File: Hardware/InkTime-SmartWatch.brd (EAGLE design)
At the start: 46 x 35 mm, 105 parts, among them IC1 BQ25180YBGR, IC2 DRV2605YZFR, IC3 BMA421, IC9 RT6160AWSC, J1 503480-2400, J2 TC2030-IDC, J4 KH-TYPE-C-16P, Q1 20V/4.2A/52mΩ/1.4W, Q3 SI1308EDL-T1-GE3, U1 NRF52840_QF, U3 MAX17048G+T10, X1 32MHz, X2 32.768kHz

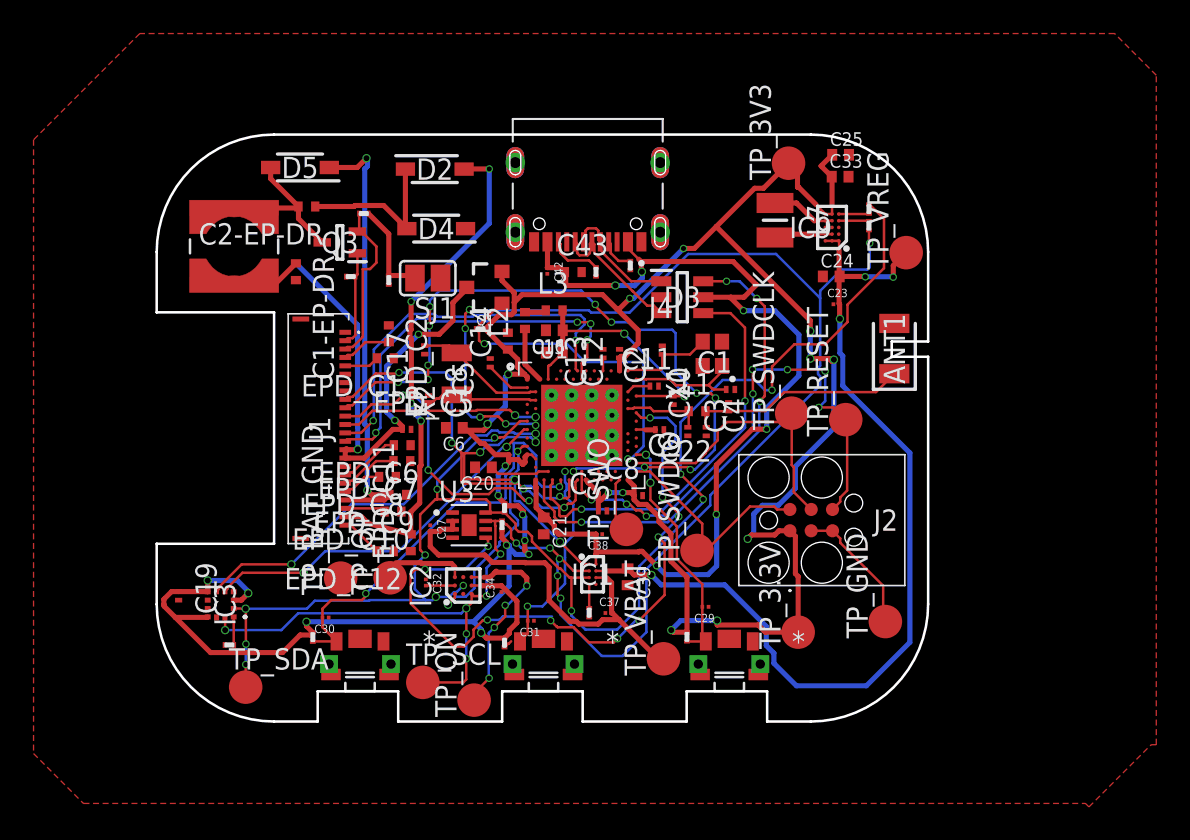
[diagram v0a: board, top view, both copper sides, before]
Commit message: Varianta finala de PCB 2D
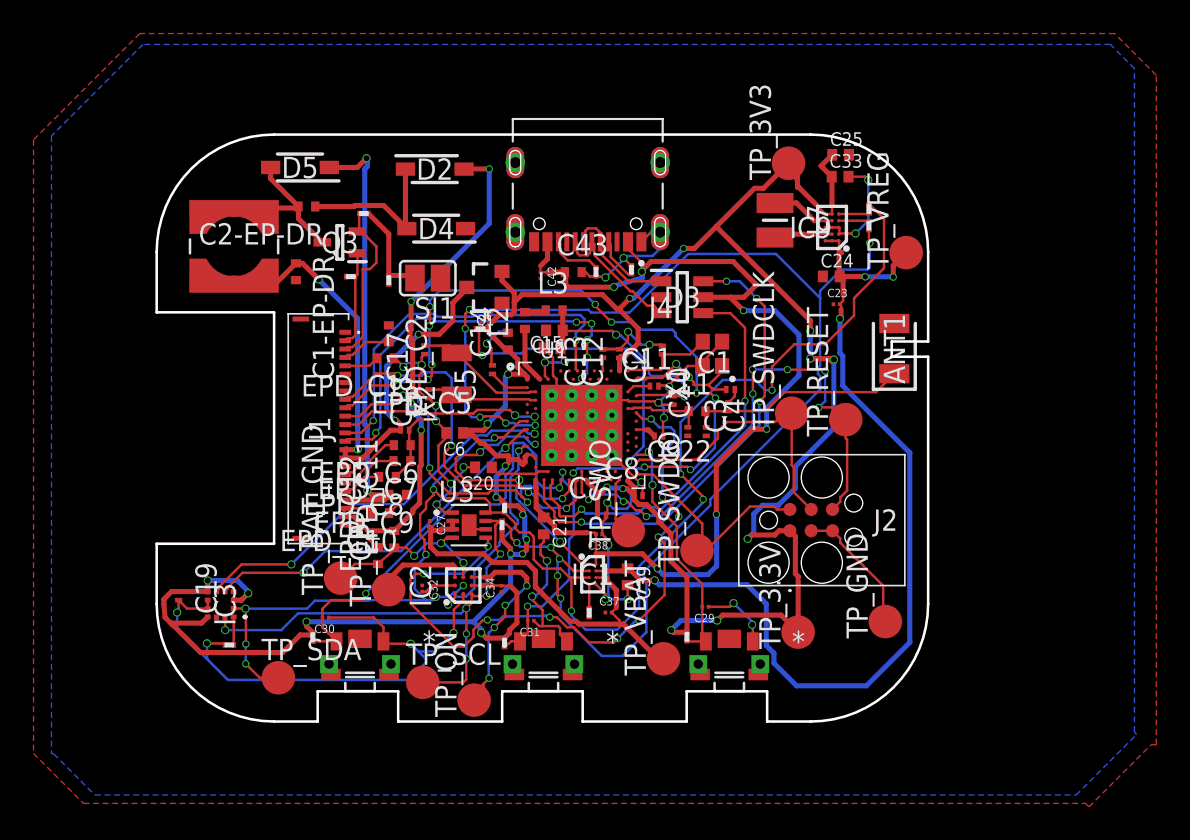
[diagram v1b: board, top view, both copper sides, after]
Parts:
- moved TP_SDA 2.03 mm to (19.0, 8.22)
- moved EPD_C11 1.00 mm to (25.9, 16.5)
- moved EPD_C10 0.74 mm to (25.1, 18.0)
- moved TP_OP 0.72 mm to (25.6, 13.5)
- moved EPD_C12 0.51 mm to (24.9, 15.5), turned to 90 degrees
- moved C42 0.49 mm to (34.7, 32.2)
- moved C5 0.43 mm to (31.8, 26.6)
- moved C32 0.42 mm to (27.6, 13.5)
- moved C9 0.38 mm to (41.7, 22.6)
- moved C18 0.36 mm to (28.0, 25.1), turned to 90 degrees
- moved C6 0.30 mm to (29.5, 22.8)
- moved C15 0.29 mm to (35.3, 27.9)
- moved C27 0.26 mm to (28.0, 17.4)
- moved R1_USB 0.26 mm to (40.1, 32.5), turned to 0 degrees
- moved C7 0.25 mm to (38.3, 17.9)
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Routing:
- net GND: track 7.01 -> 168.3 mm, vias 0 -> 33
- net 3V3: track 166.6 -> 168.9 mm
- net SDA: track 88.5 -> 90.6 mm
- net SWDIO: track 11.8 -> 13.7 mm
- net N$19: track 16.4 -> 18.1 mm, vias 2 -> 4
- net VBUS: track 58.7 -> 60.2 mm
- net N$3: track 7.11 -> 8.56 mm, vias 0 -> 2
- net OUT+: track 4.22 -> 5.57 mm
- net VREG: track 55.3 -> 56.5 mm
- net LX1: track 2.74 -> 3.92 mm
- net OUT-: track 11.4 -> 12.5 mm
- net P1.01: track 19.7 -> 20.6 mm
- net PMIC_INT: track 16.7 -> 17.5 mm
- net SWDCLK: track 16.2 -> 17.0 mm
- net N$26: track 2.43 -> 1.73 mm
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- added copper zone on layer 16, net GND
